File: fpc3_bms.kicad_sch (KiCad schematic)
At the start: 1 part

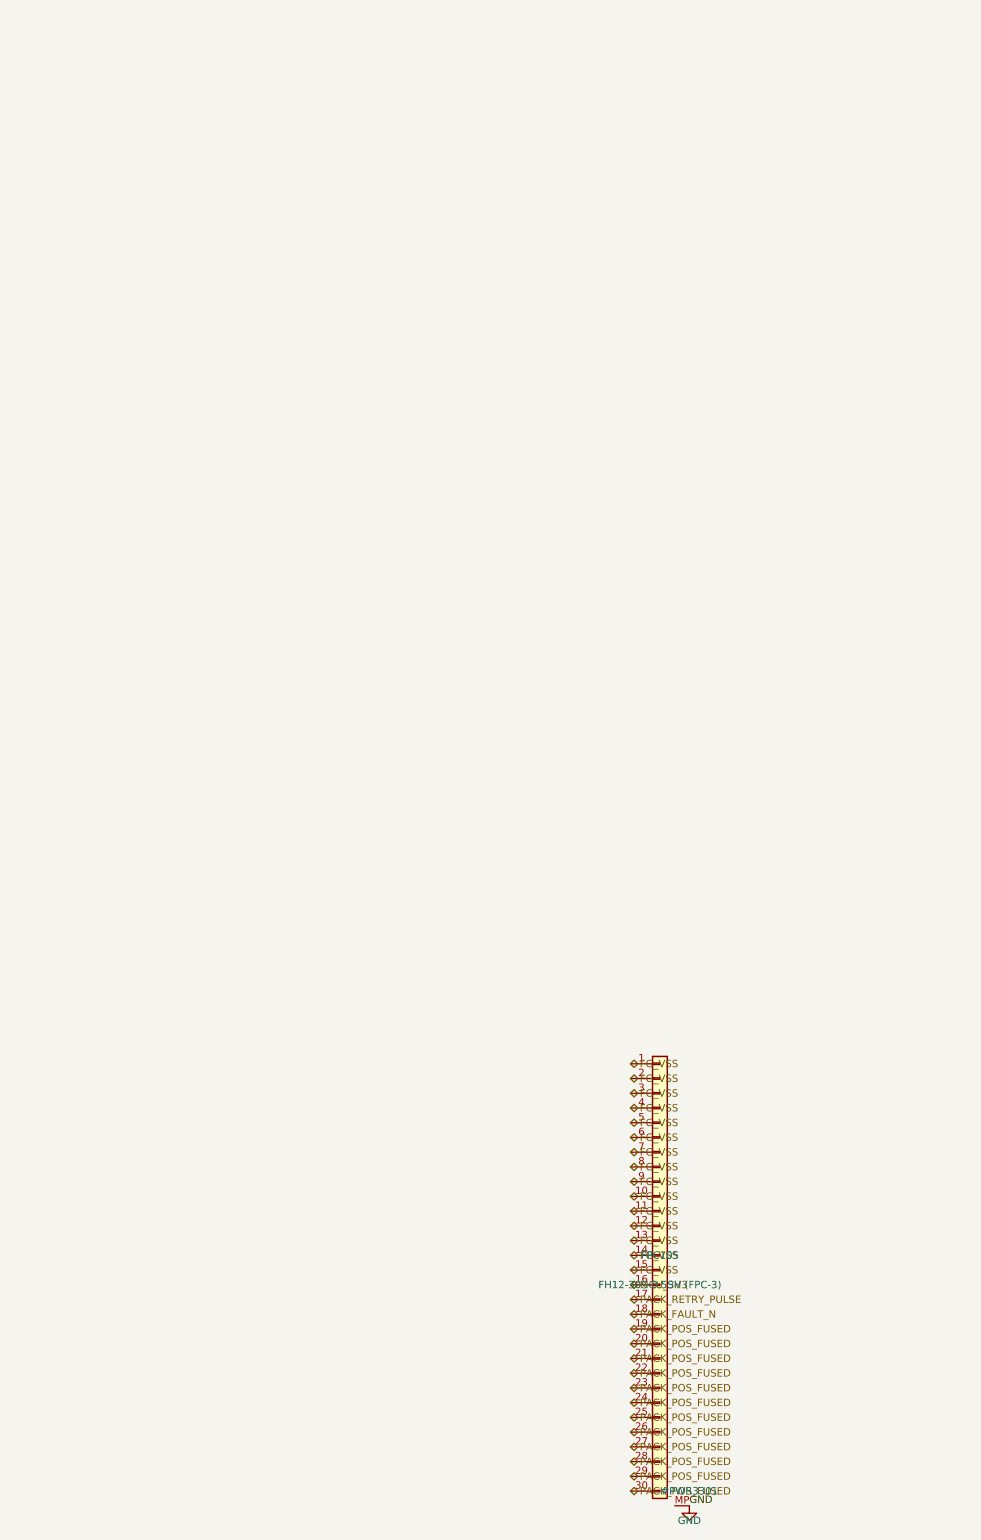
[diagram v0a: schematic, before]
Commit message: fix audit issues and move some connectors
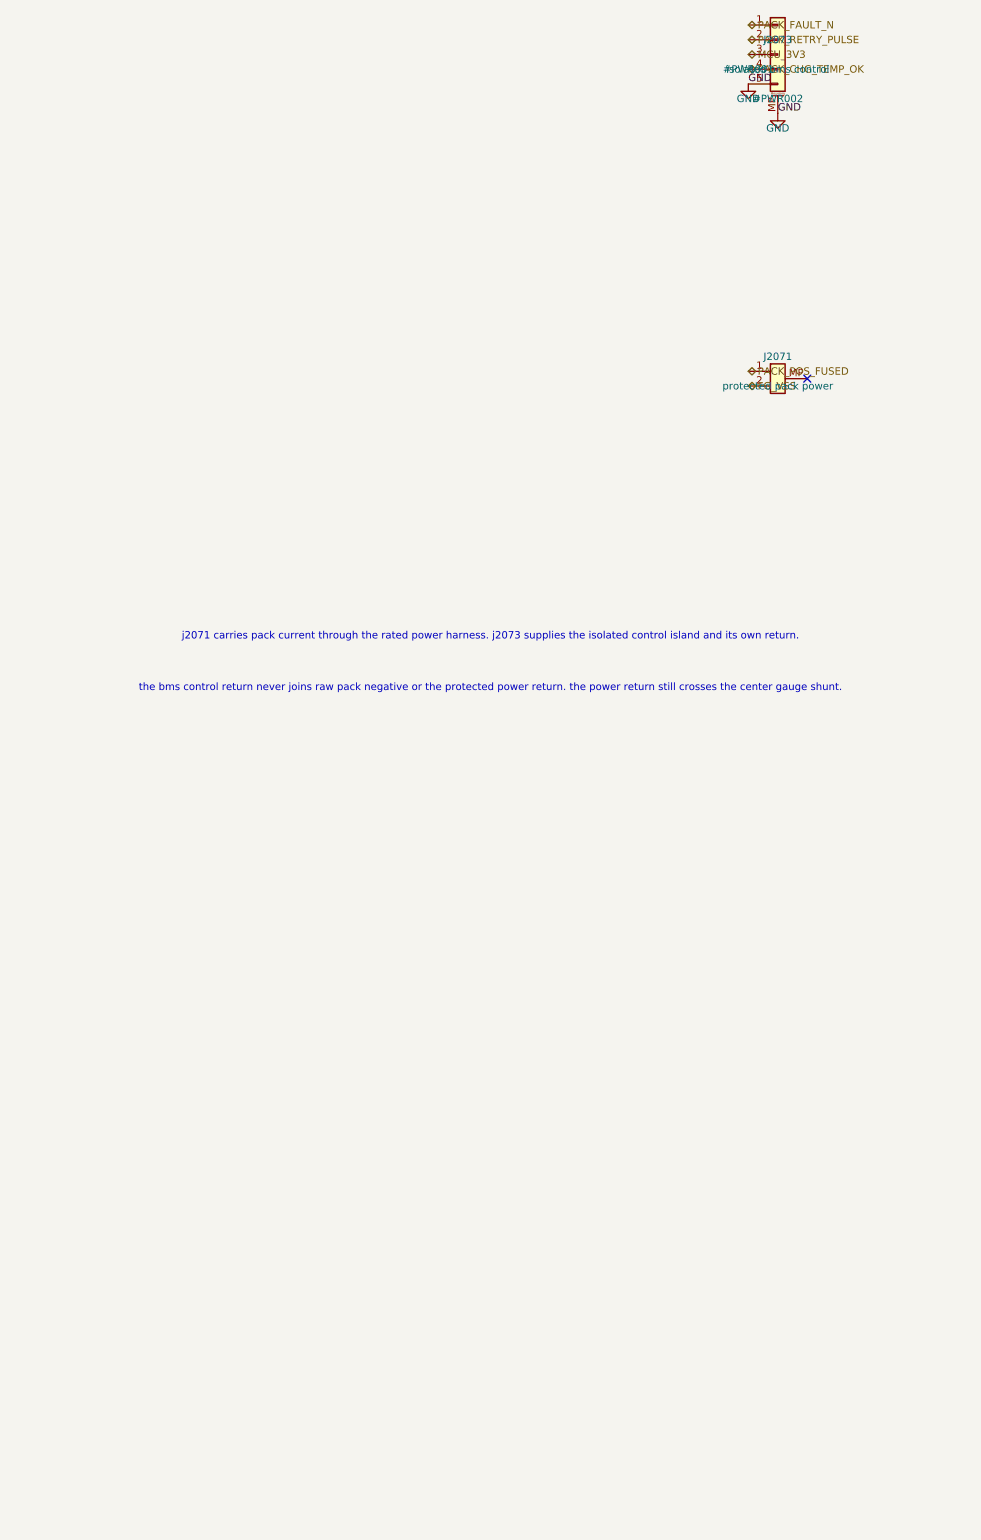
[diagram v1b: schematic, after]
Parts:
- removed FPC105: FH12-30S-0.5SH (FPC-3), Connector_FFC-FPC:Hirose_FH12-30S-0.5SH_1x30-1MP_P0.50mm_Horizontal, symbol Conn_01x30_FFC_MP:Conn_01x30_FFC_MP
- added J2071: protected pack power, Connector_Molex:Molex_Micro-Fit_3.0_43650-0224_1x02-1MP_P3.00mm_Vertical, symbol Conn_01x02_MP:Conn_01x02_MP
- added J2073: isolated bms control, Connector_JST:JST_SH_SM05B-SRSS-TB_1x05-1MP_P1.00mm_Horizontal, symbol Connector_Generic_MountingPin:Conn_01x05_MountingPin
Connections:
- net FG_VSS: now also J2071.2 (Pin_2)
- net GND: now also J2073.5 (Pin_5), J2073.MP (MountPin)
- net MCU_3V3: now also J2073.3 (Pin_3)
- net PACK_FAULT_N: now also J2073.1 (Pin_1)
- net PACK_POS_FUSED: now also J2071.1 (Pin_1)
- net PACK_RETRY_PULSE: now also J2073.2 (Pin_2)
- new net PACK_CHG_TEMP_OK: J2073.4 (Pin_4)
- no-connect marks 0 -> 1
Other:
- note added: "j2071 carries pack current through the rated power harness. j2073 supplies the isolated control island and its own return."
- note added: "the bms control return never joins raw pack negative or the protected power return. the power return still crosses the center gauge shunt."

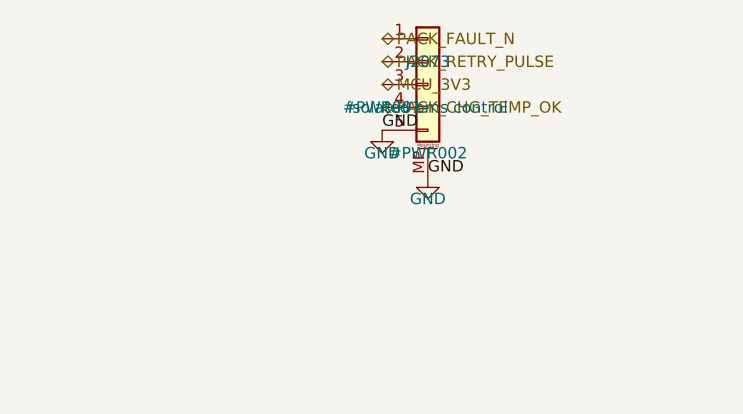
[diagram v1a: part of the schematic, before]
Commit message: fix the center layout and more board issues
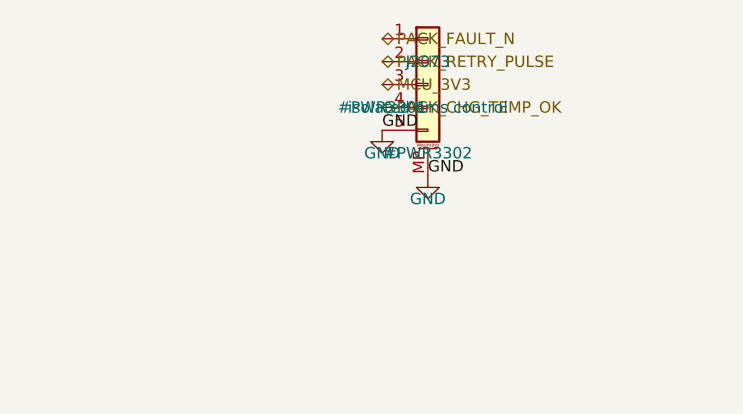
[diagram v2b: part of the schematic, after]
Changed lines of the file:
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@@
   (on_board yes)
   (dnp no)
-  (property "Reference" "#PWR001" (at 74.93 92.71 0) (effects (font (size 1.27 1.27))))
+  (property "Reference" "#PWR3301" (at 74.93 92.71 0) (effects (font (size 1.27 1.27))))
   (property "Value" "GND" (at 74.93 97.79 0) (effects (font (size 1.27 1.27))))
   (property "Footprint" "" (at 74.93 95.25 0) (effects (font (size 1.27 1.27)) (hide yes)))
@@
     (project "ducktop2"
       (path "/46b21d0a-abb0-598b-9ae3-ea30d11d7d3c"
-        (reference "#PWR001")
+        (reference "#PWR3301")
         (unit 1)
       )
@@
   (on_board yes)
   (dnp no)
-  (property "Reference" "#PWR002" (at 80.01 97.79 0) (effects (font (size 1.27 1.27))))
+  (property "Reference" "#PWR3302" (at 80.01 97.79 0) (effects (font (size 1.27 1.27))))
   (property "Value" "GND" (at 80.01 102.87 0) (effects (font (size 1.27 1.27))))
   (property "Footprint" "" (at 80.01 100.33 0) (effects (font (size 1.27 1.27)) (hide yes)))
@@
     (project "ducktop2"
       (path "/46b21d0a-abb0-598b-9ae3-ea30d11d7d3c"
-        (reference "#PWR002")
+        (reference "#PWR3302")
         (unit 1)
       )
